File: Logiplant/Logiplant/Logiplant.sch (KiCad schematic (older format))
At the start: 18 parts, among them J4 POWER, J6 Conn_RELE, J7 Conn_IMPRESOR, U2 ESP32-DEVKITC-32D

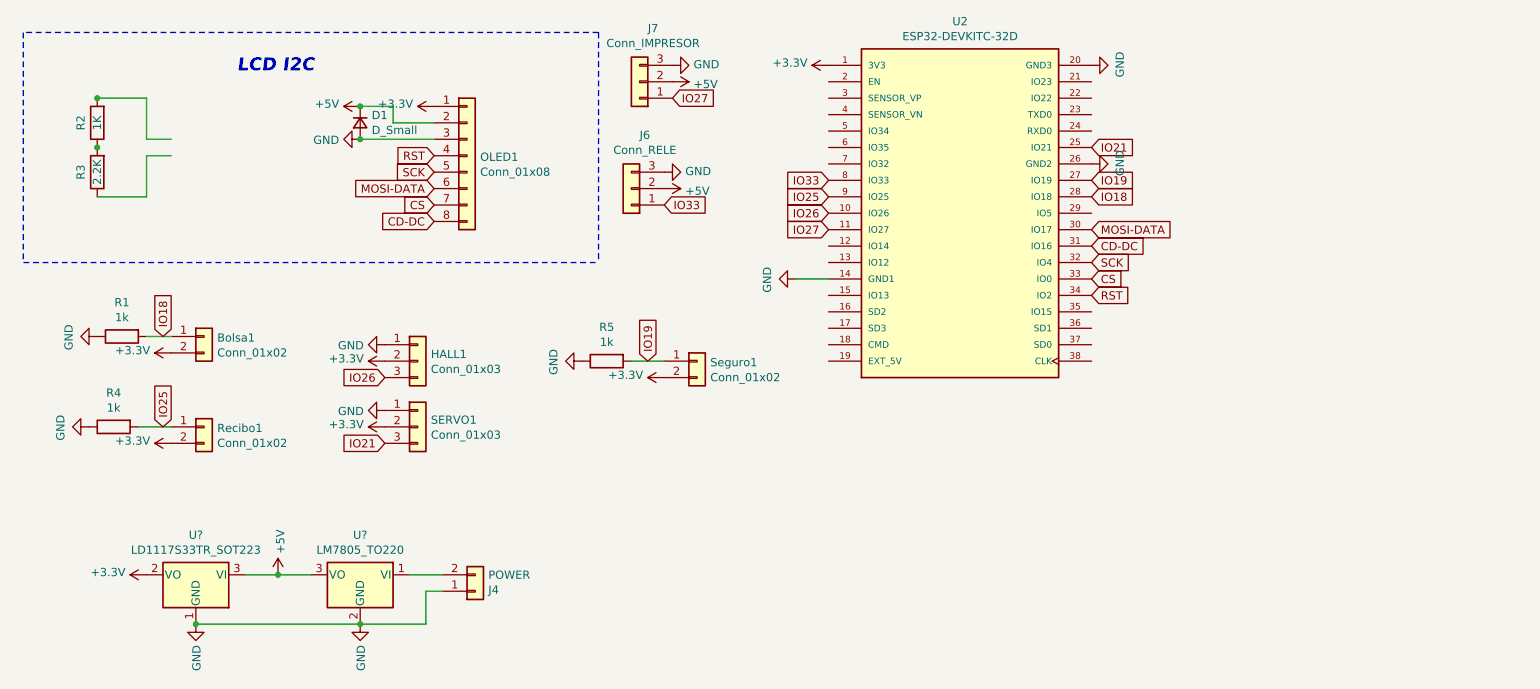
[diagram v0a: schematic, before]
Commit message: Nuevo prog
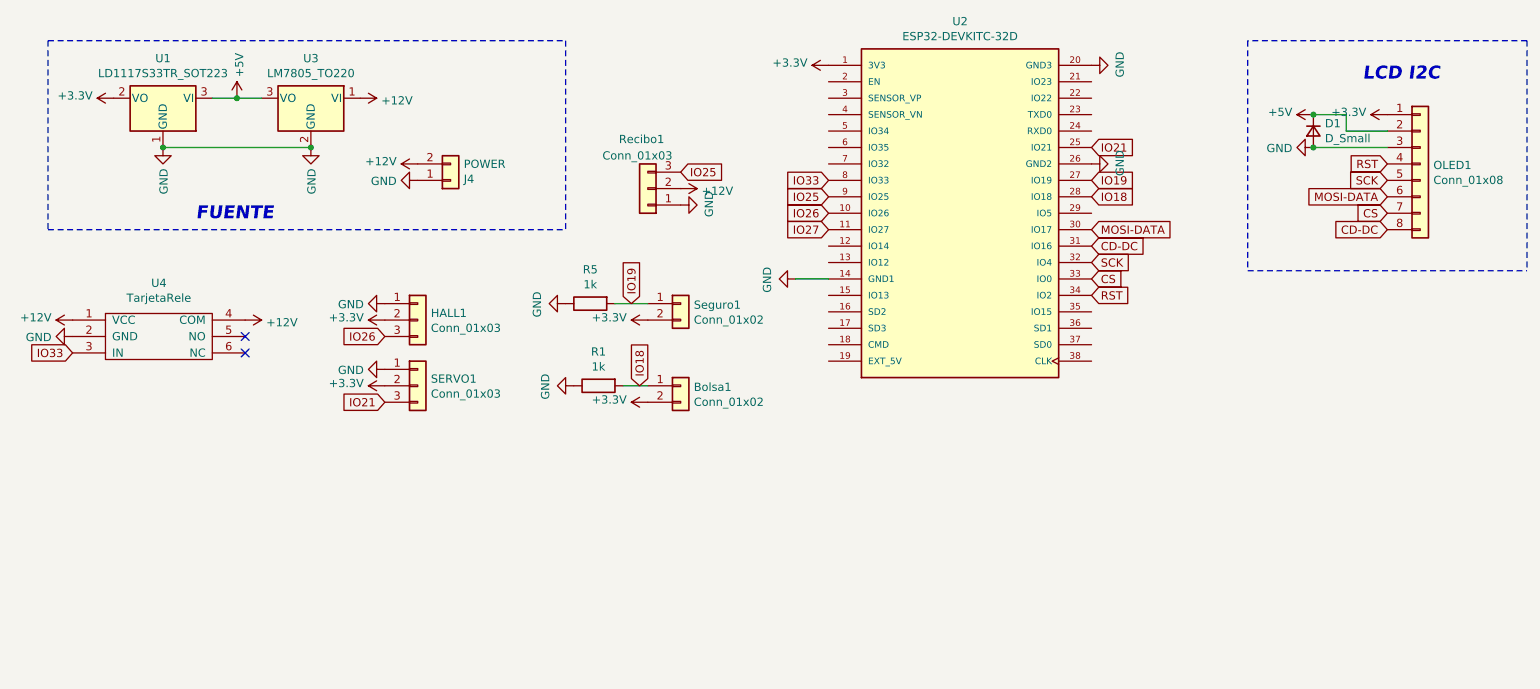
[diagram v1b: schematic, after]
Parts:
- removed J6: Conn_RELE, MODULOS:ReleYYG, symbol Connector_Generic:Conn_01x03
- removed J7: Conn_IMPRESOR, TerminalBlock_Phoenix:TerminalBlock_Phoenix_MKDS-1,5-3-5.08_1x03_P5.08mm_Horizontal, symbol Connector_Generic:Conn_01x03
- removed R2: 1K, Resistor_THT:R_Axial_DIN0207_L6.3mm_D2.5mm_P5.08mm_Vertical, symbol Device:R
- removed R3: 2.2K, Resistor_THT:R_Axial_DIN0207_L6.3mm_D2.5mm_P5.08mm_Vertical, symbol Device:R
- removed R4: 1k, Resistor_THT:R_Axial_DIN0207_L6.3mm_D2.5mm_P5.08mm_Vertical, symbol Device:R
- removed Recibo1: Conn_01x02, Connector_PinHeader_2.54mm:PinHeader_1x02_P2.54mm_Vertical, symbol Connector_Generic:Conn_01x02
- added Recibo1: Conn_01x03, TerminalBlock_Phoenix:TerminalBlock_Phoenix_MKDS-1,5-3-5.08_1x03_P5.08mm_Horizontal, symbol Connector_Generic:Conn_01x03
- added U4: TarjetaRele, MODULOS:ReleYYG, symbol TarjetaRele:TarjetaRele
- U1: renamed from U?; footprint Package_TO_SOT_SMD:SOT-223-3_TabPin2 -> Package_TO_SOT_THT:TO-220-3_Vertical
- gave numbers to parts that had none: 1
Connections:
- net labels added: +12V
- wire segments 21 -> 10
- no-connect marks 0 -> 2
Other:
- note added: "FUENTE"
- moved on the sheet: Bolsa1, D1, HALL1, J4, OLED1, R1, R5, SERVO1, Seguro1, U1, U3
